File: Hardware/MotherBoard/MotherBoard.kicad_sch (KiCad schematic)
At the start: 17 parts, among them J1 POWER, J10 I/O_PWR, J2 I/O0, J5 I/O1, J6 EXTRN_CLCK, SW2 SW_SPST, U1 AMS1117-5.0

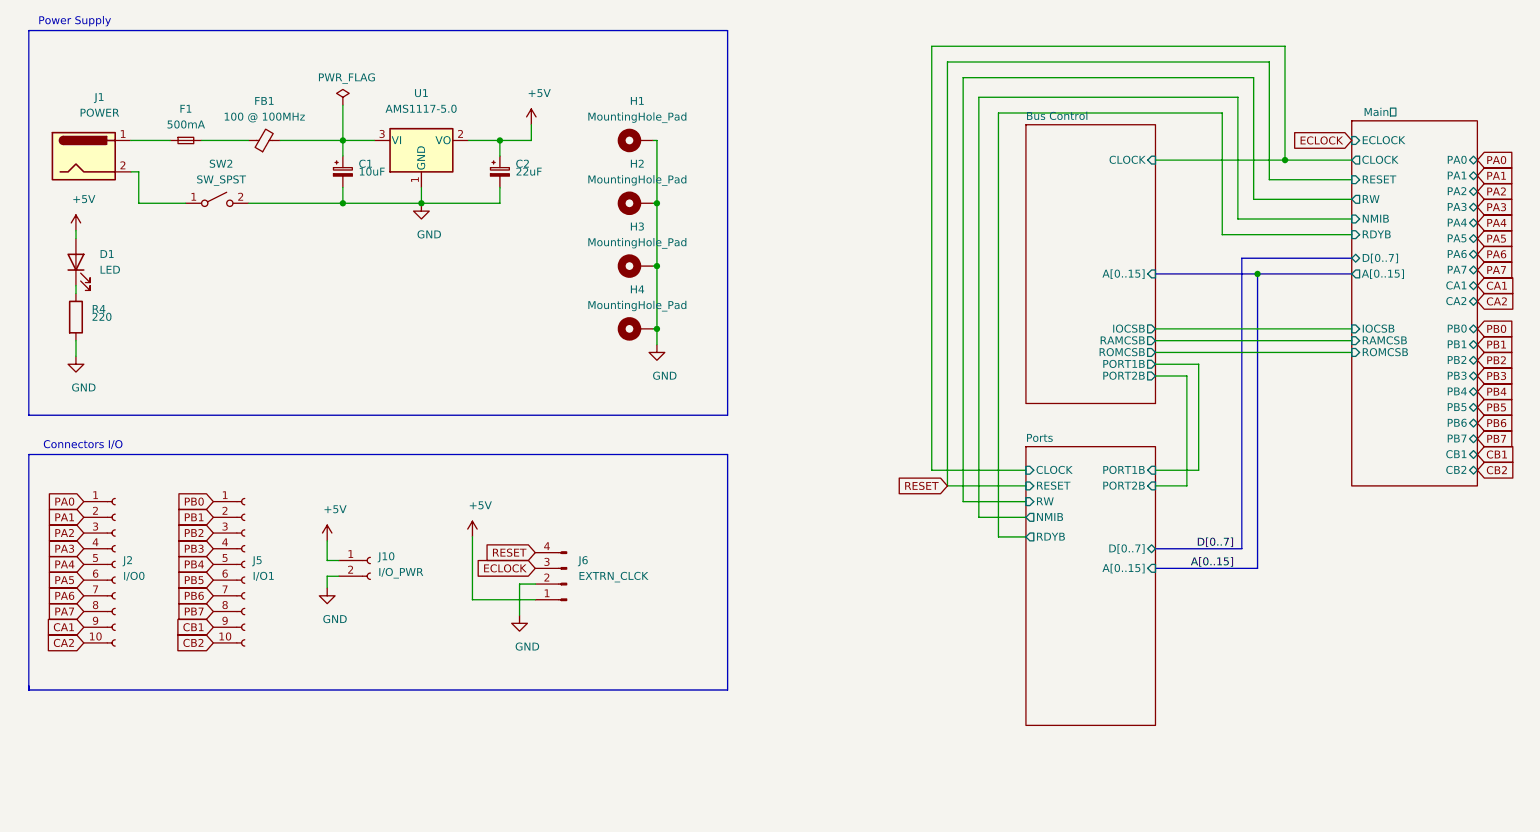
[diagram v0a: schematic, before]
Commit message: Version 1.2
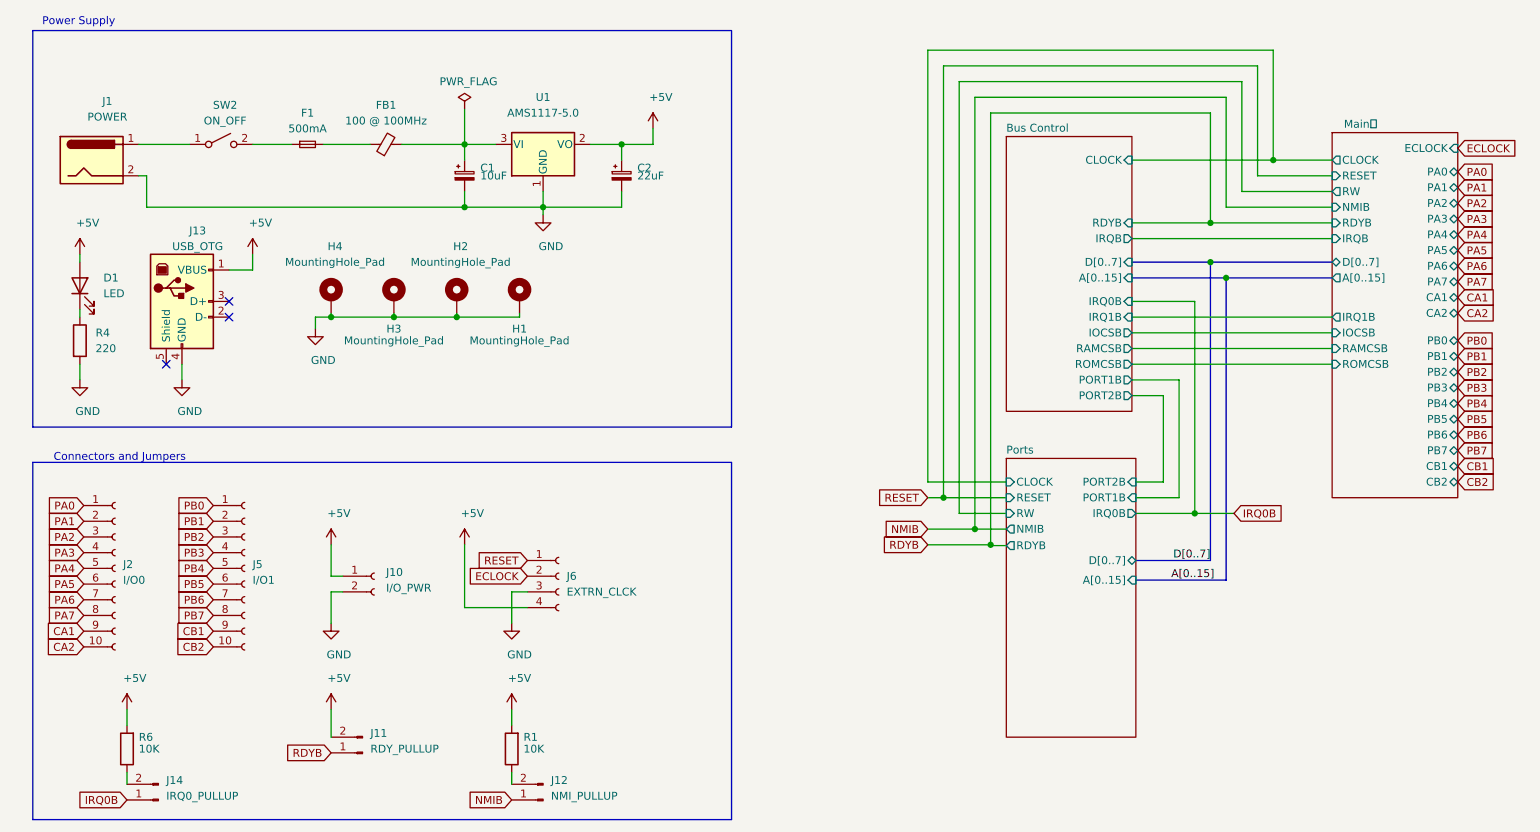
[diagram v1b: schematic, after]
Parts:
- added J11: RDY_PULLUP, Connector_PinHeader_2.54mm:PinHeader_1x02_P2.54mm_Vertical, symbol Connector:Conn_01x02_Male
- added J12: NMI_PULLUP, Connector_PinHeader_2.54mm:PinHeader_1x02_P2.54mm_Vertical, symbol Connector:Conn_01x02_Male
- added J13: USB_OTG, Connector_USB:USB_B_OST_USB-B1HSxx_Horizontal, symbol Connector:USB_B
- added J14: IRQ0_PULLUP, Connector_PinHeader_2.54mm:PinHeader_1x02_P2.54mm_Vertical, symbol Connector:Conn_01x02_Male
- added R1, R6: 10K, Resistor_THT:R_Axial_DIN0207_L6.3mm_D2.5mm_P10.16mm_Horizontal, symbol Device:R
- J6: symbol Connector:Conn_01x04_Male -> Connector:Conn_01x04_Female
- SW2: value SW_SPST -> ON_OFF
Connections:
- net +5V: now also J6.4 (Pin_4), J11.2 (Pin_2), J13.1 (VBUS), R1.2, R6.2; no longer J6.1 (Pin_1)
- net ECLOCK: now also J6.2 (Pin_2); no longer J6.3 (Pin_3)
- net GND: now also J1.2, J6.3 (Pin_3), J13.4 (GND); no longer J6.2 (Pin_2), SW2.2 (B)
- net RESET: now also J6.1 (Pin_1); no longer J6.4 (Pin_4)
- net at J1.1: now also SW2.1 (A); no longer F1.1
- new net: J12.2 (Pin_2), R1.1
- new net: J14.2 (Pin_2), R6.1
- new net: F1.1, SW2.2 (B)
- new net IRQ0B: J14.1 (Pin_1)
- new net NMIB: J12.1 (Pin_1)
- new net RDYB: J11.1 (Pin_1)
- no-connect marks 0 -> 3
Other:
- sheet Bus Control ports: added D[0..7], IRQ0B, IRQ1B, IRQB, RDYB; removed none
- sheet Main  ports: added IRQ1B, IRQB; removed none
- sheet Ports ports: added IRQ0B; removed none
- note added: "Connectors and Jumpers"
- note removed: "Connectors I/O"
- moved on the sheet: C1, C2, D1, F1, FB1, H1, H2, H3, H4, J1, J10, J2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
